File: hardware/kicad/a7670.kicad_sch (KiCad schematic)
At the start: 54 parts, among them J4 SMN-304, J5 BWIPX-1-001E, Q1 S8050, Q2 S8050, Q5 S8050, Q6 S8050, U2 A7670C_24x24mm, U5 MIC29302WU

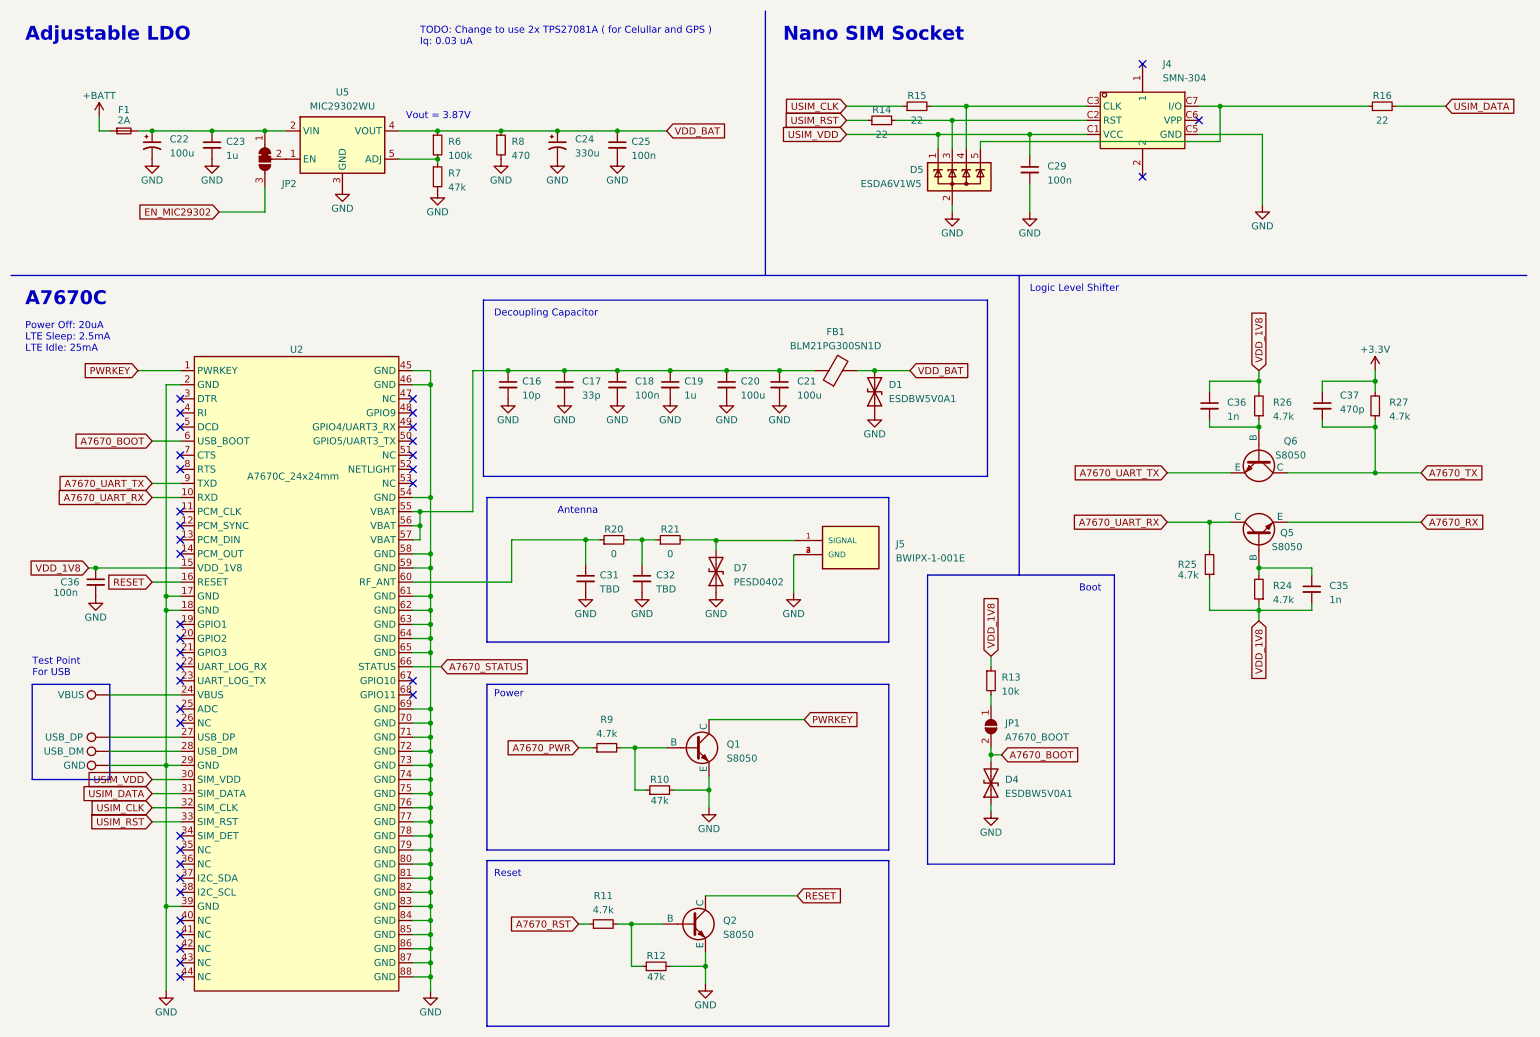
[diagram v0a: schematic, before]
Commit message: wip
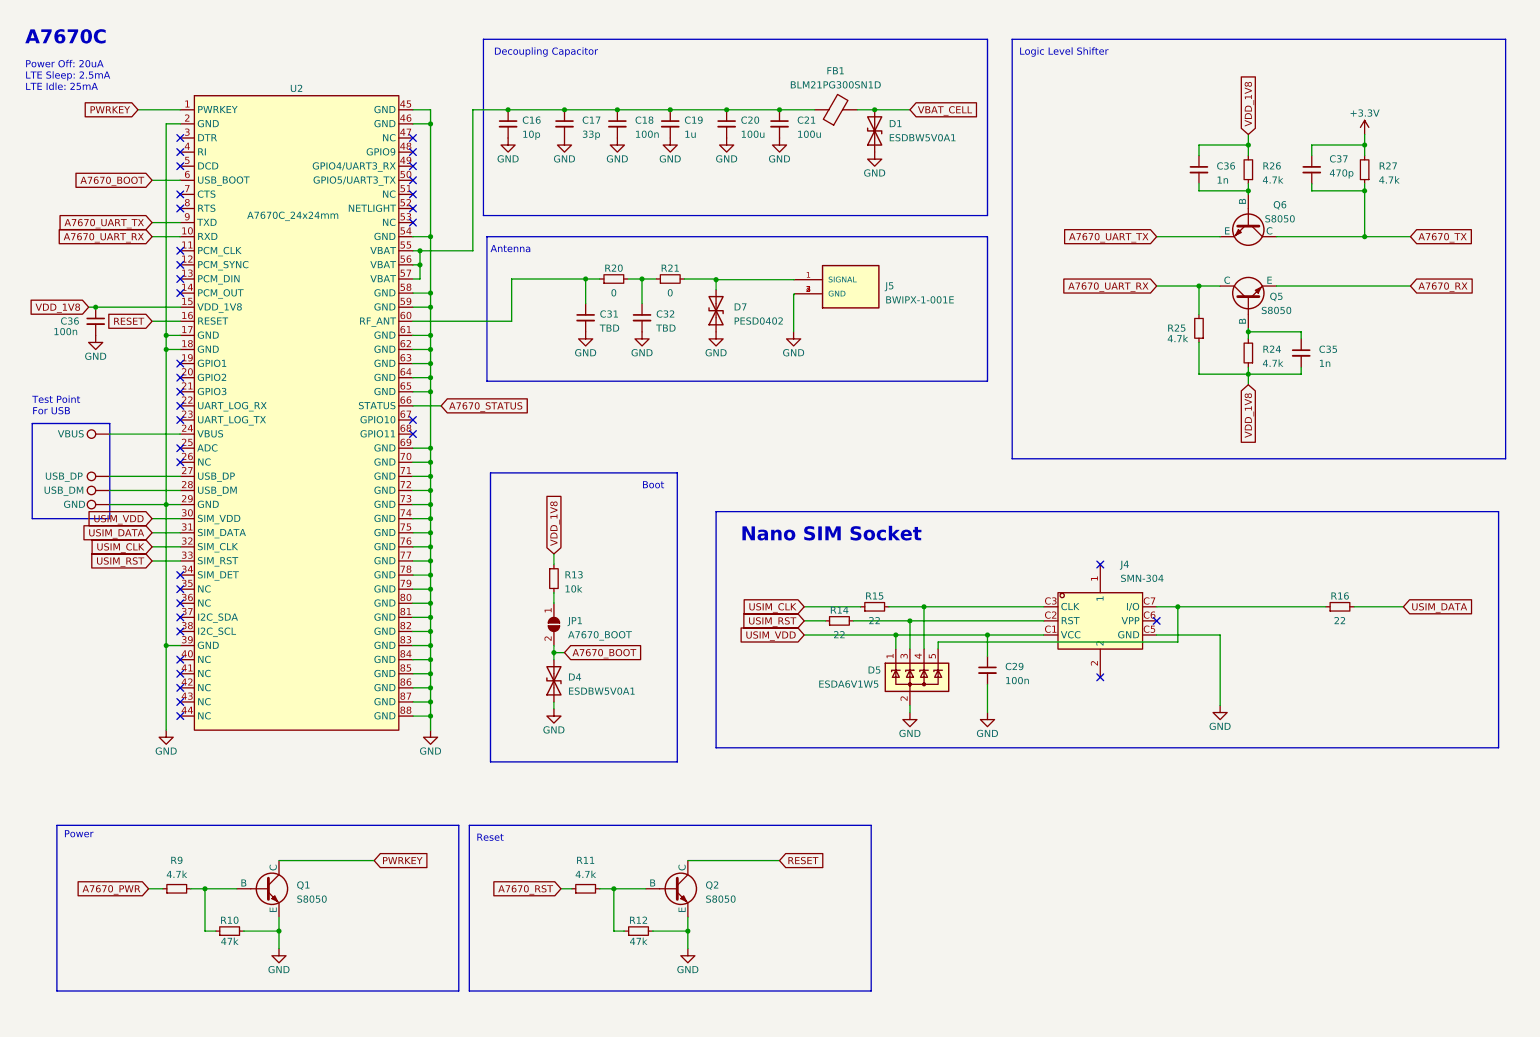
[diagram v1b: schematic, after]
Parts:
- removed C22: 100u, Capacitor_SMD:CP_Elec_6.3x5.4, symbol Device:C_Polarized_Small_US
- removed C23: 1u, Capacitor_SMD:C_0603_1608Metric, symbol Device:C_Small
- removed C24: 330u, Capacitor_SMD:CP_Elec_6.3x5.4, symbol Device:C_Polarized_Small_US
- removed C25: 100n, Capacitor_SMD:C_0805_2012Metric, symbol Device:C_Small
- removed F1: 2A, Fuse:Fuse_1812_4532Metric, symbol Device:Fuse_Small
- removed JP2: EN_MIC29302, Jumper:SolderJumper-3_P1.3mm_Bridged2Bar12_RoundedPad1.0x1.5mm, symbol Jumper:SolderJumper_3_Bridged12
- removed R6: 100k, Resistor_SMD:R_0402_1005Metric, symbol Device:R_Small
- removed R7: 47k, Resistor_SMD:R_0402_1005Metric, symbol Device:R_Small
- removed R8: 470, Resistor_SMD:R_0402_1005Metric, symbol Device:R_Small
- removed U5: MIC29302WU, Package_TO_SOT_SMD:TO-263-5_TabPin3, symbol Regulator_Linear:MIC29302WU
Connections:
- net VDD_BAT renamed VBAT_CELL
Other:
- note removed: "Adjustable LDO"
- note removed: "TODO: Change to use 2x TPS27081A ( for Celullar and GPS ) Iq: 0.03 uA"
- note removed: "Vout = 3.87V"
- moved on the sheet: C16, C17, C18, C19, C20, C21, C29, C31, C32, C35, C36, C37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

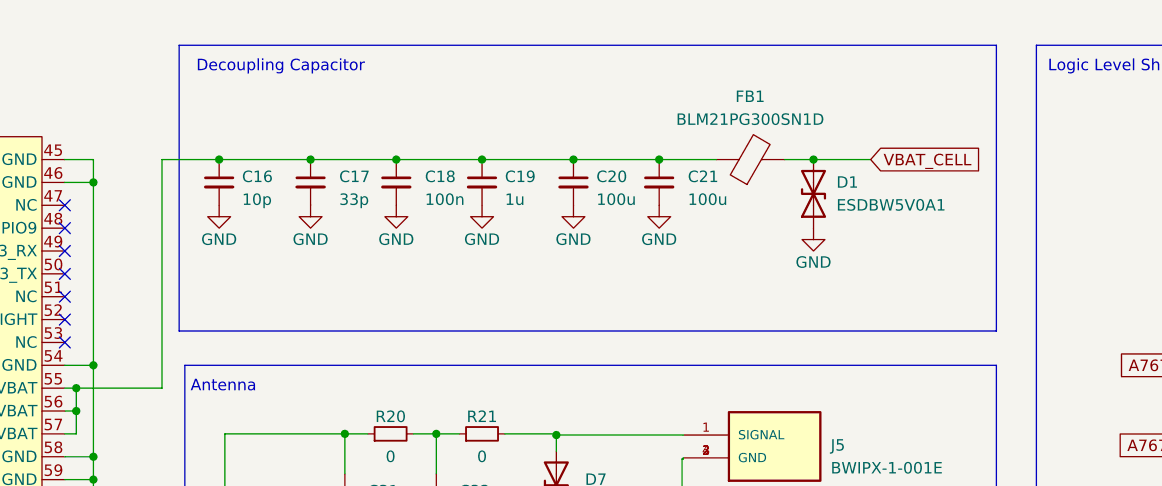
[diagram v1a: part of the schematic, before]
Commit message: wip: revision 2
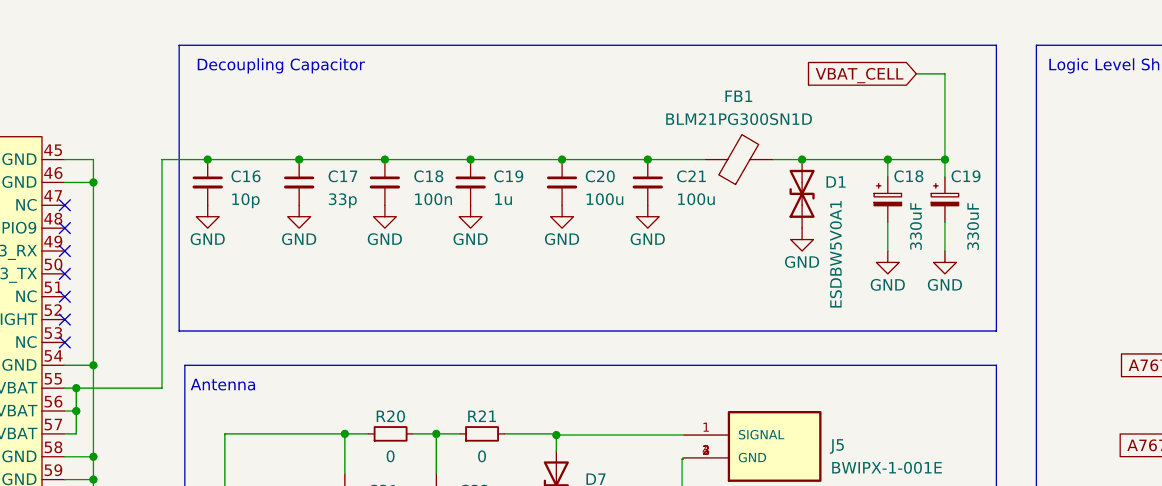
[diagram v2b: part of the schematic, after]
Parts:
- added C18, C19: 330uF, Capacitor_Tantalum_SMD:CP_EIA-3528-15_AVX-H_Pad1.50x2.35mm_HandSolder, symbol Device:C_Polarized_Small
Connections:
- net GND: now also C18.2, C19.2
- net VBAT_CELL: now also C18.1, C19.1
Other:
- moved on the sheet: C16, C17, C18, C19, C20, C21, D1, FB1

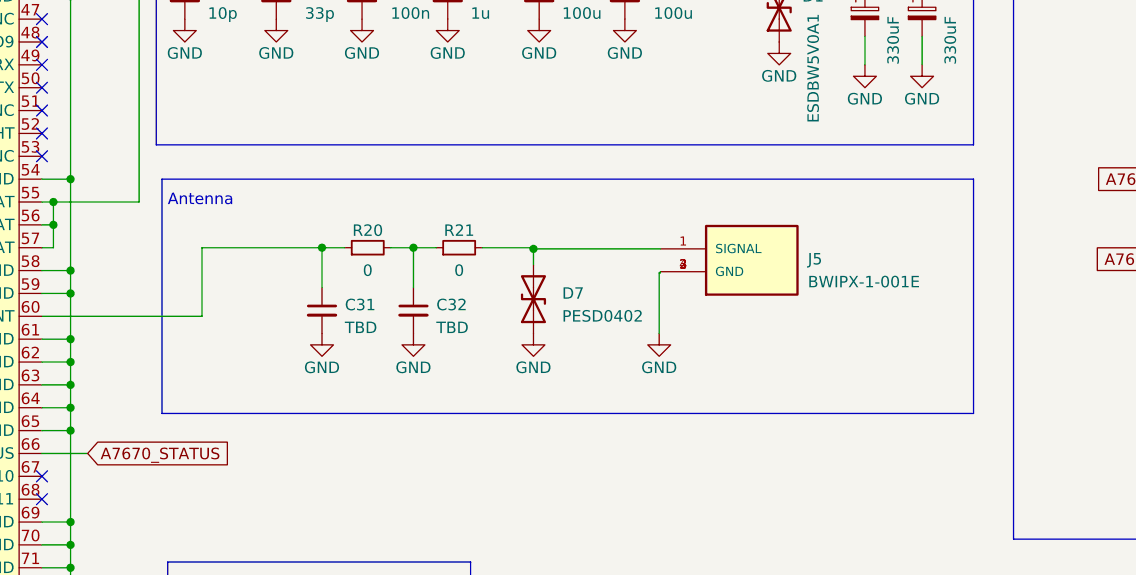
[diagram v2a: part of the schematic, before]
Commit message: wip: revision 2
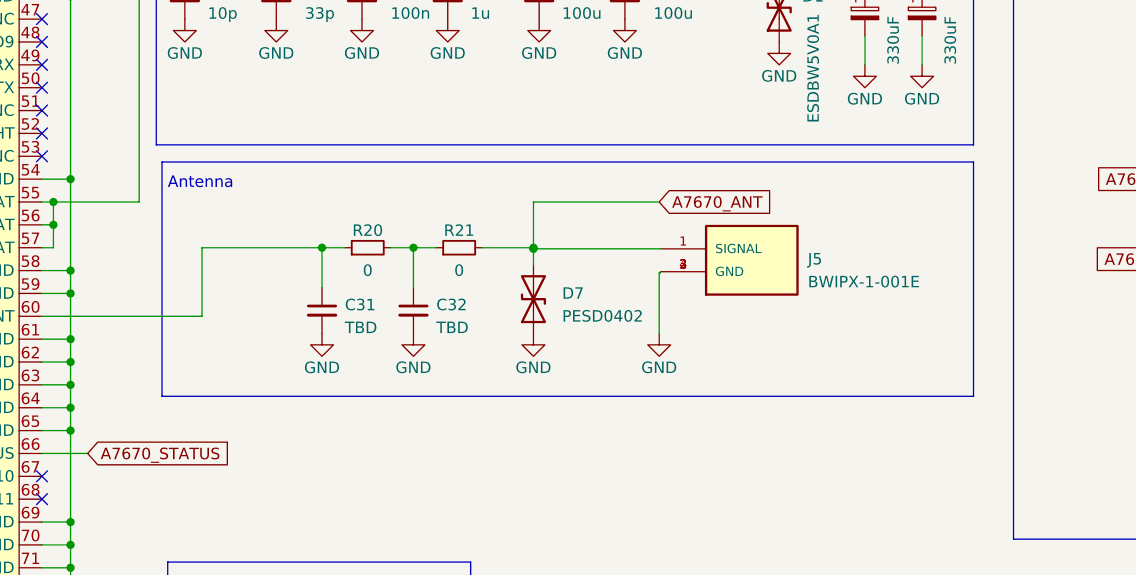
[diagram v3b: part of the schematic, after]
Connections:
- net A7670_ANT: now reaches D7.2 (A2), J5.1 (SIGNAL), R21.2
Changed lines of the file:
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@@
   (junction (at 46.99 170.18) (diameter 0) (color 0 0 0 0)
+  )
+  (junction (at 139.065 60.325) (diameter 0) (color 0 0 0 0)
   )
   (junction (at 133.985 177.8) (diameter 0) (color 0 0 0 0)
@@
     (stroke (width 0) (type default))
   )
+  (wire (pts (xy 153.035 55.245) (xy 139.065 55.245))
+    (stroke (width 0) (type default))
+  )
   (wire (pts (xy 226.06 36.195) (xy 234.95 36.195))
     (stroke (width 0) (type default))
@@
     (stroke (width 0) (type default))
   )
+  (wire (pts (xy 139.065 55.245) (xy 139.065 60.325))
+    (stroke (width 0) (type default))
+  )
   (wire (pts (xy 255.905 52.705) (xy 255.905 44.45))
     (stroke (width 0) (type default))
@@
     (fill (type none))
   )
-  (rectangle (start 97.79 52.705) (end 187.96 78.74)
+  (rectangle (start 97.79 50.8) (end 187.96 76.835)
     (stroke (width 0) (type default))
     (fill (type none))
@@
     (effects (font (size 1.27 1.27)) (justify left bottom))
   )
-  (text "Antenna" (at 98.425 55.88 0)
+  (text "Antenna" (at 98.425 53.975 0)
     (effects (font (size 1.27 1.27)) (justify left bottom))
   )
@@
     )
   )
+  (global_label "A7670_ANT" (shape input) (at 153.035 55.245 0) (fields_autoplaced)
+    (effects (font (size 1.27 1.27)) (justify left))
+    (property "Intersheetrefs" "${INTERSHEET_REFS}" (at 166.2217 55.245 0)
+      (effects (font (size 1.27 1.27)) (justify left) hide)
+    )
+  )
